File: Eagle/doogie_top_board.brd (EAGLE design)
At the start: 92.9 x 75 mm, 18 parts, among them T1 BC337, U1 GY-521MPU6050, U2 U1V10F5, U3 74HC4051_SPARKFUN

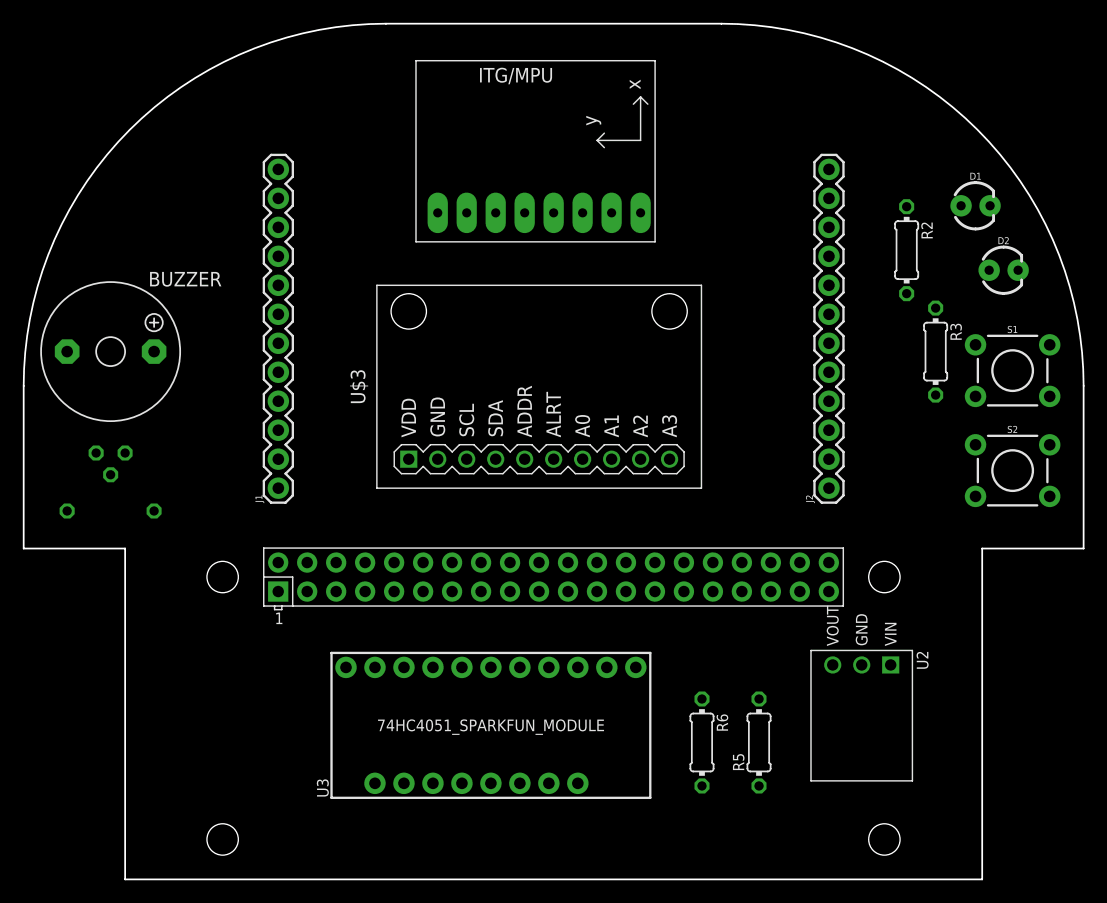
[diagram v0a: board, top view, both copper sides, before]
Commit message: Make top board routing sketch
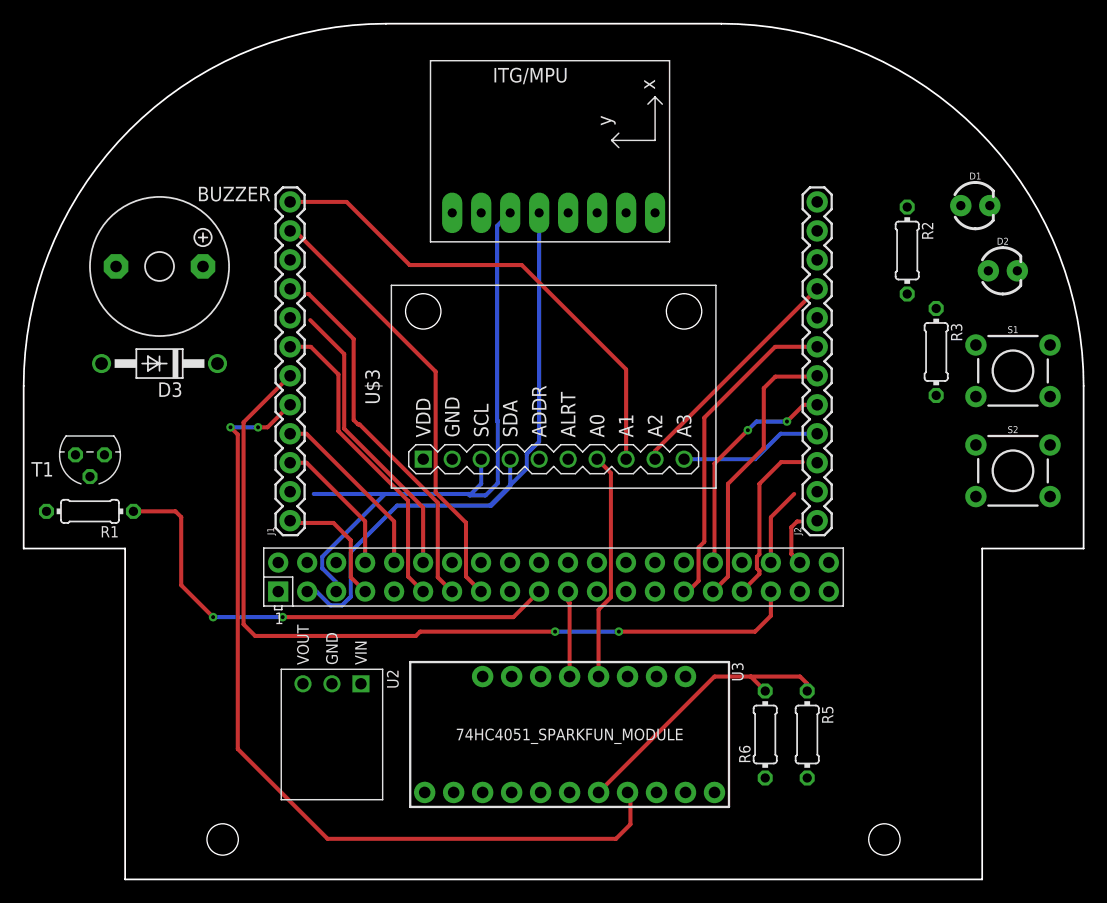
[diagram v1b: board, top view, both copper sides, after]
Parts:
- added D3: 1N4004, diode:DO41-10
- U$2: device RPI-Zero:RASPBERRYPI_BASTELSTUBE_V13_RASPI_BOARD_B+_FULL -> doogie:RASPBERRYPI_BASTELSTUBE_V13_RASPI_BOARD_B+_FULL
- moved U2 46.5 mm to (-19.4, 12.7)
- moved BUZZER 8.60 mm to (-34.5, 53.7)
- moved U3 6.94 mm to (1.40, 12.7), turned to 270 degrees
- moved R6 5.59 mm to (18.5, 12.7), turned to 90 degrees
- moved R5 4.28 mm to (22.2, 12.7), turned to 270 degrees
- moved J1 3.03 mm to (-23.1, 31.4)
- moved J2 3.03 mm to (23.1, 31.4)
- moved T1 1.82 mm to (-40.6, 37.2), flipped to the top
- moved R1 1.81 mm to (-40.6, 32.3), flipped to the top, turned to 180 degrees
- moved U$3 1.27 mm to (0.00, 43.2)
- moved U1 1.27 mm to (0.00, 67.3)
- moved D2 0.09 mm to (39.4, 53.3)
- moved R3 0.06 mm to (33.5, 46.2)
- moved R2 0.06 mm to (31.0, 55.1)
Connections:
- removed net GND@7: U$2.14, U$2.20, U$2.30, U$2.34, U$2.6
- net 5V: now also D3.C
- net GND: now also J1.10, J2.8, S1.3, S2.3, U$2.14, U$2.20, U$2.30, U$2.34, U$2.6; no longer J1.6, S1.1, S2.1
- net H-BRIDGE_!STDBY: now also J1.9, U$2.13; no longer J1.7, U$2.11
- net LEFT_EMITTER_CTRL: now also U$2.7; no longer U$2.10
- net MOTOR_LEFT_EN1: now also J1.8, U$2.12; no longer J1.9, U$2.13
- net MOTOR_LEFT_EN2: now also J1.7, U$2.11; no longer J1.8, U$2.12
- net MOTOR_LEFT_ENCA: now also J1.3; no longer J1.4
- net MOTOR_LEFT_ENCB: now also J1.4, U$2.10; no longer J1.3, U$2.7
- net MOTOR_LEFT_PWM: now also J1.6; no longer J1.10
- net MOTOR_RIGHT_EN1: now also J2.7, U$2.29; no longer J2.6, U$2.36
- net MOTOR_RIGHT_EN2: now also J2.6, U$2.31; no longer J2.5, U$2.37
- net MOTOR_RIGHT_ENCA: now also U$2.36; no longer U$2.38
- net MOTOR_RIGHT_ENCB: now also U$2.38; no longer U$2.40
- net MOTOR_RIGHT_PWM: now also J2.5; no longer J2.7
- net N$1: now also D3.A
- net N$3: now also S2.1, U$2.37; no longer S2.3, U$2.33
- net N$4: now also S1.1, U$2.40; no longer S1.3, U$2.31
- net RIGHT_EMITTER_CTRL: now also U$2.33; no longer U$2.28
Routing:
- net LEFT_RCVR: track 0.00 -> 75.6 mm, vias 0 -> 2
- net MOTOR_LEFT_PWM: track 0.00 -> 73.0 mm, vias 0 -> 2
- net I2C_SCL: track 0.00 -> 55.9 mm
- net I2C_SDA: track 0.00 -> 54.8 mm
- net BUZZER_CTRL: track 0.00 -> 43.8 mm, vias 0 -> 2
- net LEFT_FRONT_RCVR: track 0.00 -> 43.4 mm
- net FRONT_EMITTERS_CTRL: track 0.00 -> 38.8 mm
- net H-BRIDGE_!STDBY: track 0.00 -> 31.5 mm
- net MOTOR_RIGHT_EN1: track 0.00 -> 28.6 mm
- net MOTOR_LEFT_EN2: track 0.00 -> 27.3 mm
- net MOTOR_LEFT_EN1: track 0.00 -> 25.4 mm
- net N$9: track 0.00 -> 25.2 mm
- net MOTOR_RIGHT_EN2: track 0.00 -> 24.8 mm
- net RIGHT_FRONT_RCVR: track 0.00 -> 20.8 mm
- net ADC_A0_CHANNEL: track 0.00 -> 20.0 mm
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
